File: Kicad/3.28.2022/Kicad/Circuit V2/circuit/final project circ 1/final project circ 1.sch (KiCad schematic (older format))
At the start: 79 parts, among them J11 Conn_01x03_Female, J14 Barrel_Jack, J2 Conn_01x01_Female, J7 Conn_01x03_Female, Q1 FDD770N15A, Q2 FDD770N15A, Q3 FDD770N15A, Q4 BC337, Q6 2SC1945, U1 LTC3895IFE, U2 ESP32-DEVKITC-32D, U3 SN74LVC2G06DCKR, U4 A4988_STEPPER_MOTOR_DRIVER_CA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, U5 AZ1117-3.3, U6 A4988_STEPPER_MOTOR_DRIVER_CA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, U7 SRD-S-112DM, U8 L2293QTR, U9 A4988_STEPPER_MOTOR_DRIVER_CA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

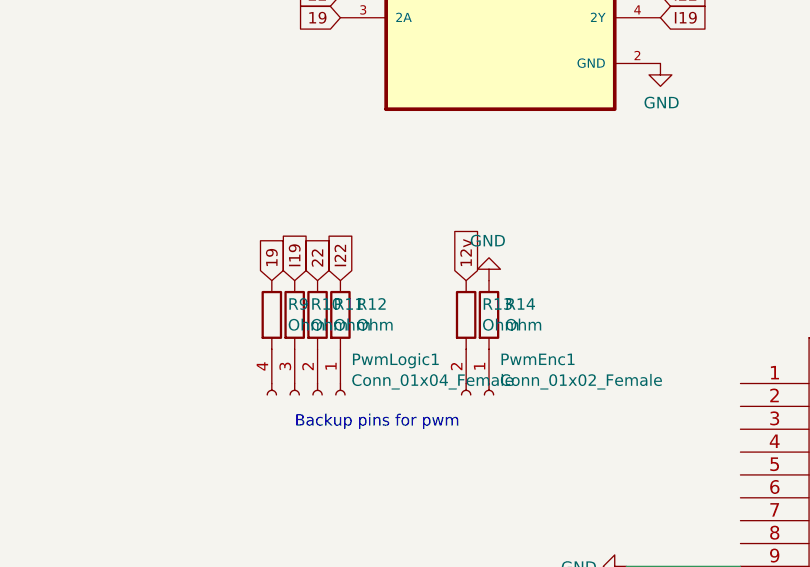
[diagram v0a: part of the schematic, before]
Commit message: update
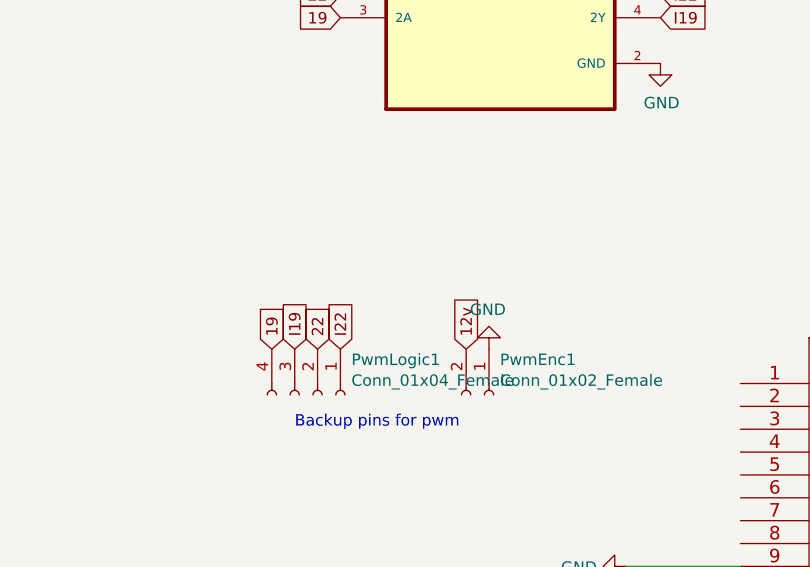
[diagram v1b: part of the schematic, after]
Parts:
- removed R10, R11, R12, R13, R14, R9: Ohm, symbol Device:R
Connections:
- net 12v: now also PwmEnc1.2 (Pin_2)
- net 19: now also PwmLogic1.4 (Pin_4)
- net 22: now also PwmLogic1.2 (Pin_2)
- net GND: now also PwmEnc1.1 (Pin_1)
- net I19: now also PwmLogic1.3 (Pin_3)
- net I22: now also PwmLogic1.1 (Pin_1)
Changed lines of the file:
@@
 	0    1    1    0
 $EndComp
-Text GLabel 20250 17000 1    50   Input ~ 0
+Text GLabel 20250 17300 1    50   Input ~ 0
 19
-Text GLabel 20350 17000 1    50   Input ~ 0
+Text GLabel 20350 17300 1    50   Input ~ 0
 I19
-Text GLabel 20450 17000 1    50   Input ~ 0
+Text GLabel 20450 17300 1    50   Input ~ 0
 22
-Text GLabel 20550 17000 1    50   Input ~ 0
+Text GLabel 20550 17300 1    50   Input ~ 0
 I22
-Text GLabel 21100 17000 1    50   Input ~ 0
+Text GLabel 21100 17300 1    50   Input ~ 0
 12v
 $Comp
 L power:GND #PWR034
 U 1 1 625004AD
-P 21200 17000
-F 0 "#PWR034" H 21200 16750 50  0001 C CNN
-F 1 "GND" H 21205 16827 50  0000 C CNN
-F 2 "" H 21200 17000 50  0001 C CNN
-F 3 "" H 21200 17000 50  0001 C CNN
-	1    21200 17000
+P 21200 17300
+F 0 "#PWR034" H 21200 17050 50  0001 C CNN
+F 1 "GND" H 21205 17127 50  0000 C CNN
+F 2 "" H 21200 17300 50  0001 C CNN
+F 3 "" H 21200 17300 50  0001 C CNN
+	1    21200 17300
 	-1   0    0    1
 $EndComp
@@
 Wire Wire Line
 	23850 12650 23750 12650
-$Comp
-L Device:R R9
-U 1 1 62785939
-P 20250 17150
-F 0 "R9" H 20320 17196 50  0000 L CNN
-F 1 "Ohm" H 20320 17105 50  0000 L CNN
-F 2 "" V 20180 17150 50  0001 C CNN
-F 3 "~" H 20250 17150 50  0001 C CNN
-	1    20250 17150
-	1    0    0    -1
-$EndComp
-$Comp
-L Device:R R10
-U 1 1 627A6606
-P 20350 17150
-F 0 "R10" H 20420 17196 50  0000 L CNN
-F 1 "Ohm" H 20420 17105 50  0000 L CNN
-F 2 "" V 20280 17150 50  0001 C CNN
-F 3 "~" H 20350 17150 50  0001 C CNN
-	1    20350 17150
-	1    0    0    -1
-$EndComp
-$Comp
-L Device:R R11
-U 1 1 627B60B0
-P 20450 17150
-F 0 "R11" H 20520 17196 50  0000 L CNN
-F 1 "Ohm" H 20520 17105 50  0000 L CNN
-F 2 "" V 20380 17150 50  0001 C CNN
-F 3 "~" H 20450 17150 50  0001 C CNN
-	1    20450 17150
-	1    0    0    -1
-$EndComp
-$Comp
-L Device:R R12
-U 1 1 627C5D43
-P 20550 17150
-F 0 "R12" H 20620 17196 50  0000 L CNN
-F 1 "Ohm" H 20620 17105 50  0000 L CNN
-F 2 "" V 20480 17150 50  0001 C CNN
-F 3 "~" H 20550 17150 50  0001 C CNN
-	1    20550 17150
-	1    0    0    -1
-$EndComp
-$Comp
-L Device:R R13
-U 1 1 627D5AAE
-P 21100 17150
-F 0 "R13" H 21170 17196 50  0000 L CNN
-F 1 "Ohm" H 21170 17105 50  0000 L CNN
-F 2 "" V 21030 17150 50  0001 C CNN
-F 3 "~" H 21100 17150 50  0001 C CNN
-	1    21100 17150
-	1    0    0    -1
-$EndComp
-$Comp
-L Device:R R14
-U 1 1 627E5621
-P 21200 17150
-F 0 "R14" H 21270 17196 50  0000 L CNN
-F 1 "Ohm" H 21270 17105 50  0000 L CNN
-F 2 "" V 21130 17150 50  0001 C CNN
-F 3 "~" H 21200 17150 50  0001 C CNN
-	1    21200 17150
-	1    0    0    -1
-$EndComp
 Wire Wire Line
 	18100 20700 18000 20700
